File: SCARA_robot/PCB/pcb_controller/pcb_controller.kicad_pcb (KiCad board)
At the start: 2 copper layers, 50 parts, among them J1 Barrel_Jack_Switch, J10 interface, J11 Conn_01x07_Socket, J12 Encoder_A, J13 Encoder_B, J14 Encoder_C, J15 Conn_01x04_Pin_STEPPER_B, J16 Conn_01x04_Pin_STEPPER_C, J2 Conn_01x04_Pin_STEPPER_A, J3 interface, J4 power, J5 Conn_01x07_Socket, J6 power, J7 interface, J8 Conn_01x07_Socket, J9 power, SW1 Microstep mode, SW2 Microstep mode, SW3 Microstep mode, U1 LM7805CT, U2 ESP32-DEVKIT-V1, U3 PCA9548A, U4 LD1117S33TR_SOT223

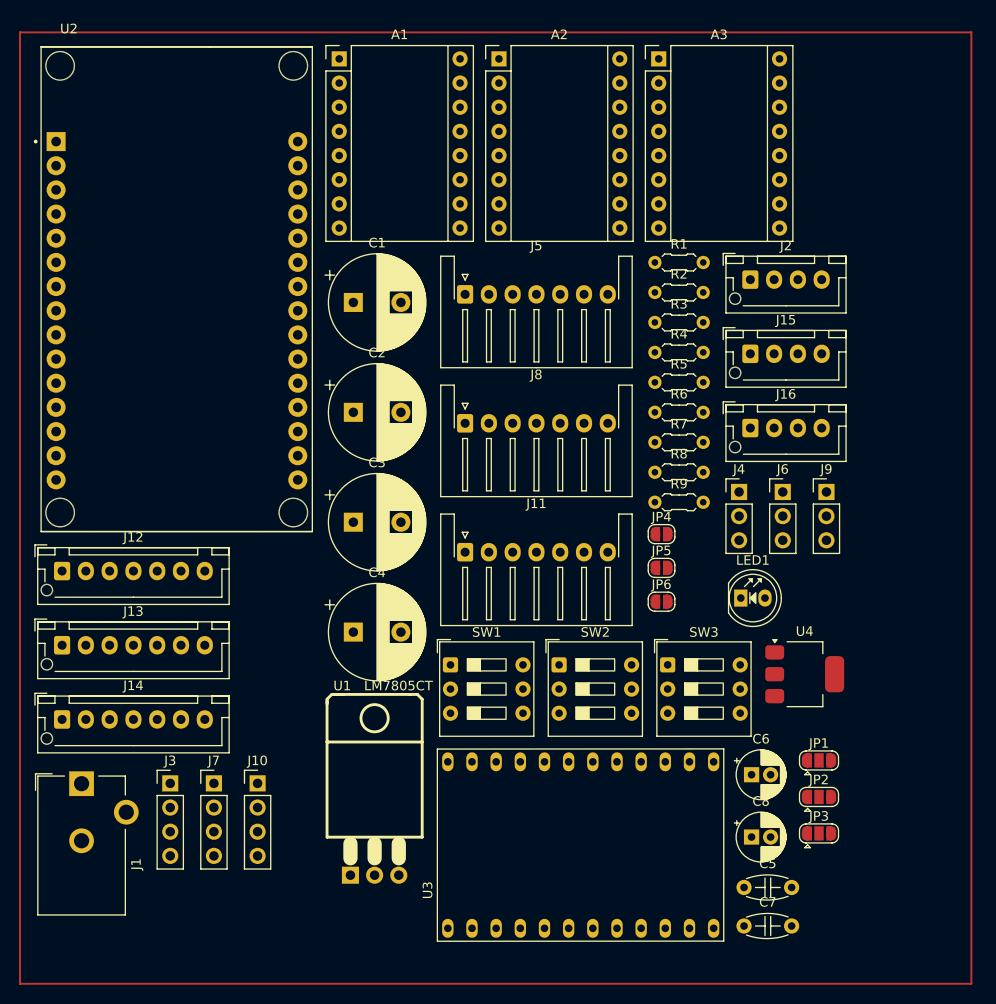
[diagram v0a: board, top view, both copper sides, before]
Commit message: pcb designed phase 1
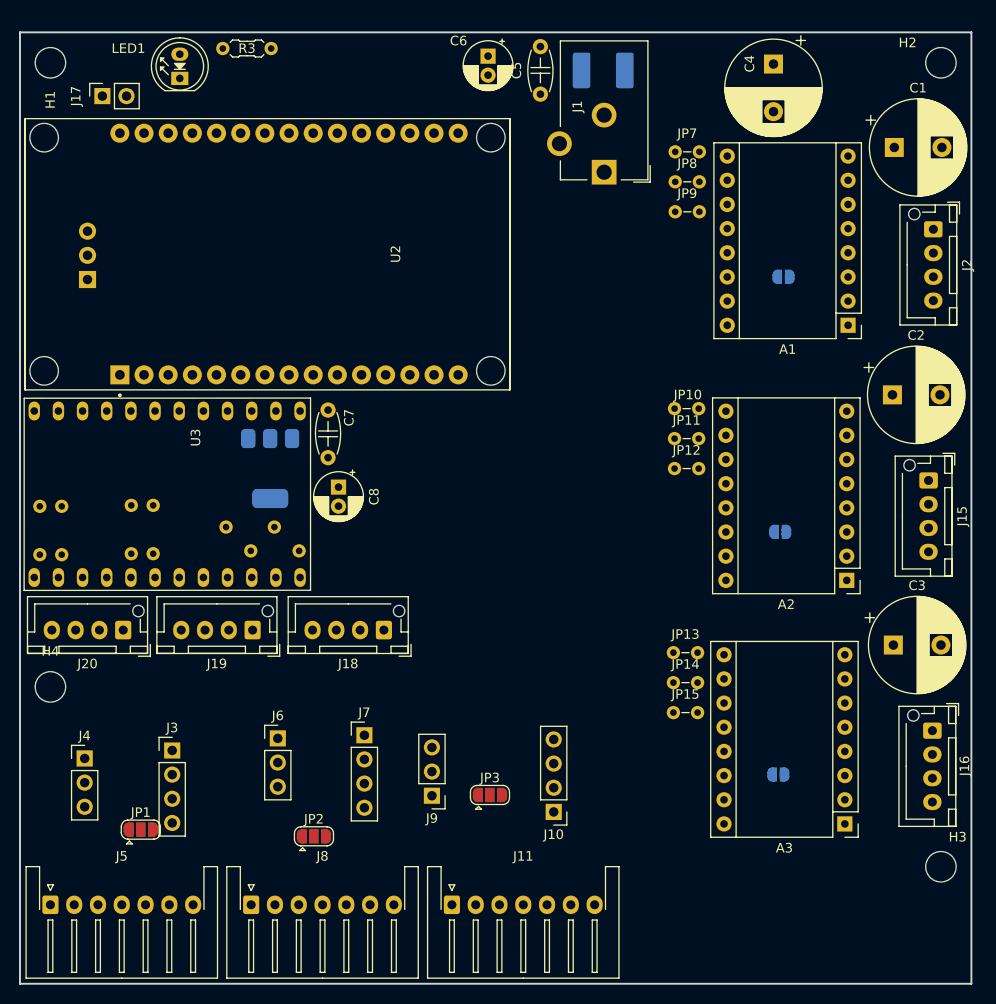
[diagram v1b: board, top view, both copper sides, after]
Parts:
- removed J12: Encoder_A, Connector_JST:JST_XH_B7B-XH-AM_1x07_P2.50mm_Vertical
- removed J13: Encoder_B, Connector_JST:JST_XH_B7B-XH-AM_1x07_P2.50mm_Vertical
- removed J14: Encoder_C, Connector_JST:JST_XH_B7B-XH-AM_1x07_P2.50mm_Vertical
- removed R1, R2: 4K7, PCM_Resistor_THT_AKL:R_Axial_DIN0204_L3.6mm_D1.6mm_P5.08mm_Horizontal
- removed SW1, SW2, SW3: Microstep mode, Button_Switch_THT:SW_DIP_SPSTx03_Slide_9.78x9.8mm_W7.62mm_P2.54mm
- added D2: SS36, Diode_SMD:D_2114_3652Metric_Pad1.85x3.75mm_HandSolder, B.Cu at (138.6, 38.1)
- added H1: MountingHole, MountingHole:MountingHole_3.2mm_M3_ISO14580, F.Cu at (80.5, 37.3)
- added H2: MountingHole, MountingHole:MountingHole_3.2mm_M3_ISO14580, F.Cu at (174.1, 37.3)
- added H3: MountingHole, MountingHole:MountingHole_3.2mm_M3_ISO14580, F.Cu at (174.1, 121.8)
- added H4: MountingHole, MountingHole:MountingHole_3.2mm_M3_ISO14580, F.Cu at (80.5, 102.9)
- added J17: Conn_01x02_Pin, Connector_PinSocket_2.54mm:PinSocket_1x02_P2.54mm_Vertical, F.Cu at (86.0, 40.8)
- added J18: Conn_01x04_Pin_STEPPER_C, Connector_JST:JST_XH_B4B-XH-AM_1x04_P2.50mm_Vertical, F.Cu at (115.5, 96.9)
- added J19: Conn_01x04_Pin_STEPPER_C, Connector_JST:JST_XH_B4B-XH-AM_1x04_P2.50mm_Vertical, F.Cu at (101.8, 96.9)
- added J20: Conn_01x04_Pin_STEPPER_C, Connector_JST:JST_XH_B4B-XH-AM_1x04_P2.50mm_Vertical, F.Cu at (88.2, 96.9)
- added JP10: Jumper_2_Open, PCM_Jumper_AKL:Jumper_P2.54mm_D0.7mm, F.Cu at (146.1, 73.7)
- added JP11: Jumper_2_Open, PCM_Jumper_AKL:Jumper_P2.54mm_D0.7mm, F.Cu at (146.1, 76.8)
- added JP12: Jumper_2_Open, PCM_Jumper_AKL:Jumper_P2.54mm_D0.7mm, F.Cu at (146.1, 80.0)
- added JP13: Jumper_2_Open, PCM_Jumper_AKL:Jumper_P2.54mm_D0.7mm, F.Cu at (146.0, 99.3)
- added JP14: Jumper_2_Open, PCM_Jumper_AKL:Jumper_P2.54mm_D0.7mm, F.Cu at (146.0, 102.5)
- added JP15: Jumper_2_Open, PCM_Jumper_AKL:Jumper_P2.54mm_D0.7mm, F.Cu at (146.0, 105.6)
- added JP7: Jumper_2_Open, PCM_Jumper_AKL:Jumper_P2.54mm_D0.7mm, F.Cu at (146.2, 46.7)
- added JP8: Jumper_2_Open, PCM_Jumper_AKL:Jumper_P2.54mm_D0.7mm, F.Cu at (146.2, 49.8)
- added JP9: Jumper_2_Open, PCM_Jumper_AKL:Jumper_P2.54mm_D0.7mm, F.Cu at (146.2, 53.0)
- JP4, JP5, JP6, R4, R5, R6, R7, R8, R9, U1, U4: moved to B.Cu
- moved C5 86.1 mm to (132.0, 40.6), turned to 90 degrees
- moved J1 84.5 mm to (138.7, 48.8), turned to 180 degrees
- moved A3 82.8 mm to (164.0, 117.3), turned to 180 degrees
- moved C6 80.4 mm to (126.5, 36.6), turned to -90 degrees
- moved LED1 80.4 mm to (94.1, 38.9), turned to 90 degrees
- moved J5 77.6 mm to (80.5, 125.8)
- moved J4 74.3 mm to (84.1, 110.4)
- moved C4 74.3 mm to (156.5, 37.4), turned to -90 degrees
- moved U1 71.8 mm to (84.4, 57.5), turned to 90 degrees
- moved JP1 71.7 mm to (90.0, 117.9)
- moved C7 69.7 mm to (109.7, 73.8), turned to -90 degrees
- moved A2 65.9 mm to (164.2, 91.7), turned to 180 degrees
- moved R9 64.6 mm to (79.4, 83.9), turned to -90 degrees
- moved U3 63.6 mm to (92.8, 77.9), turned to 180 degrees
- moved R8 62.5 mm to (81.7, 83.9), turned to -90 degrees
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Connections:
- J1 pad 1: +12V -> Net-(D2-A)
- J15 pad 3: Net-(A2-A2) -> Net-(A2-A1)
- J15 pad 4: Net-(A2-A1) -> Net-(A2-A2)
- J16 pad 3: Net-(A3-A2) -> Net-(A3-A1)
- J16 pad 4: Net-(A3-A1) -> Net-(A3-A2)
- J2 pad 3: Net-(A1-A2) -> Net-(A1-A1)
- J2 pad 4: Net-(A1-A1) -> Net-(A1-A2)
- U2 pad 30: +5V -> Net-(J17-Pin_2)
- U3 pad 15: /scl_enB -> unconnected-(U3-sc6-Pad15)
- U3 pad 16: /sda_enB -> unconnected-(U3-sd6-Pad16)
- U3 pad 17: /scl_enC -> unconnected-(U3-sc5-Pad17)
- U3 pad 18: /sda_enC -> unconnected-(U3-sd5-Pad18)
- U3 pad 19: unconnected-(U3-sc4-Pad19) -> /scl_enB
- U3 pad 20: unconnected-(U3-sd4-Pad20) -> /sda_enB
- U3 pad 23: unconnected-(U3-sc2-Pad23) -> /scl_enC
- U3 pad 24: unconnected-(U3-sd2-Pad24) -> /sda_enC
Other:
- board outline added: 100 x 100 mm
